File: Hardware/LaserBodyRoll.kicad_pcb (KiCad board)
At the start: 2 copper layers, 104 x 40 mm, 93 parts, among them J1 CONN_01X02, J2 FTSH-105-01-L-DV-K, J3 Conn_01x04, J4 Conn_01x04, J5 CONN_01X02, J6 CONN_01X02, J8 Raspberry_Pi_2_3, Q1 Q_NPN_BCE, Q2 Q_NPN_BCE, Q3 Q_NPN_BCE, Q4 Q_NPN_BCE, U1 TPS821XX, U2 CY8C4A25LQI-473, U3 LMC6032, U5 ICM-20602, U6 VL53L0X, U7 STLM75

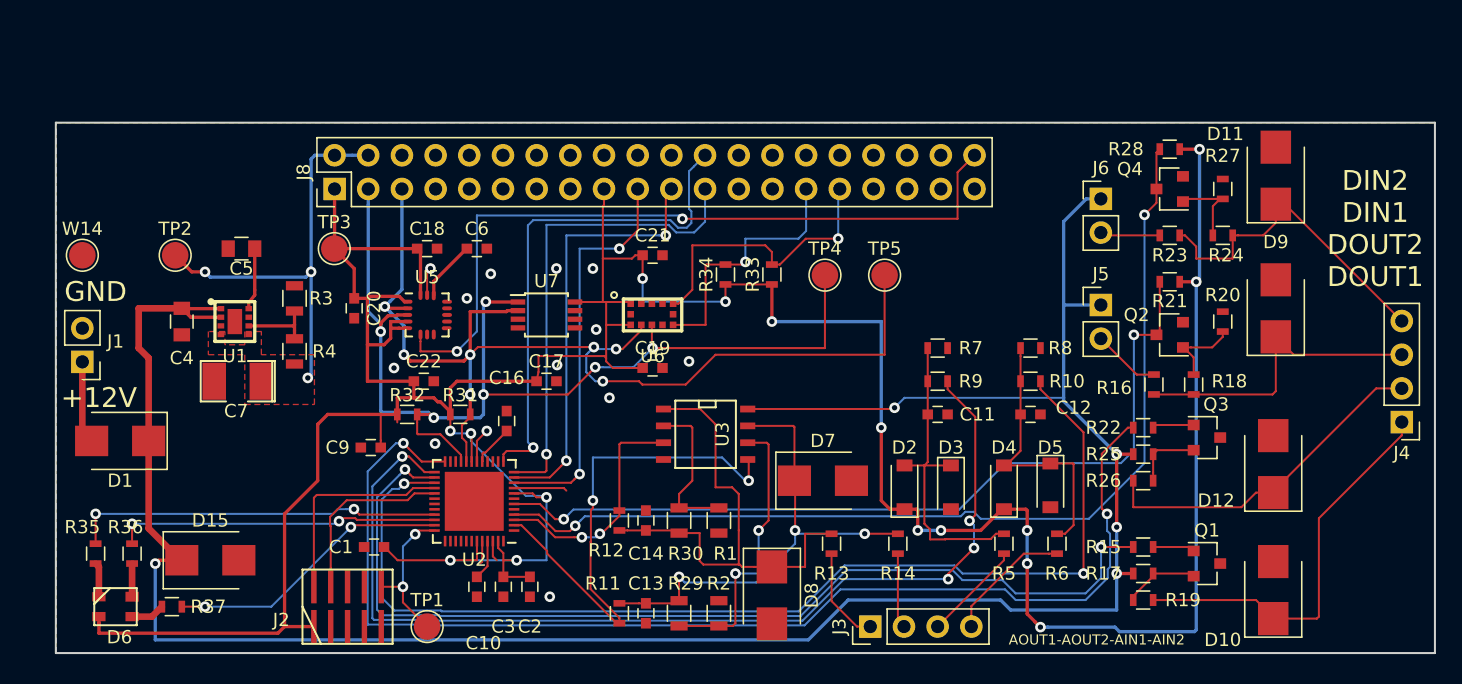
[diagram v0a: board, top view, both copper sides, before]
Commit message: Worked on initial placement.
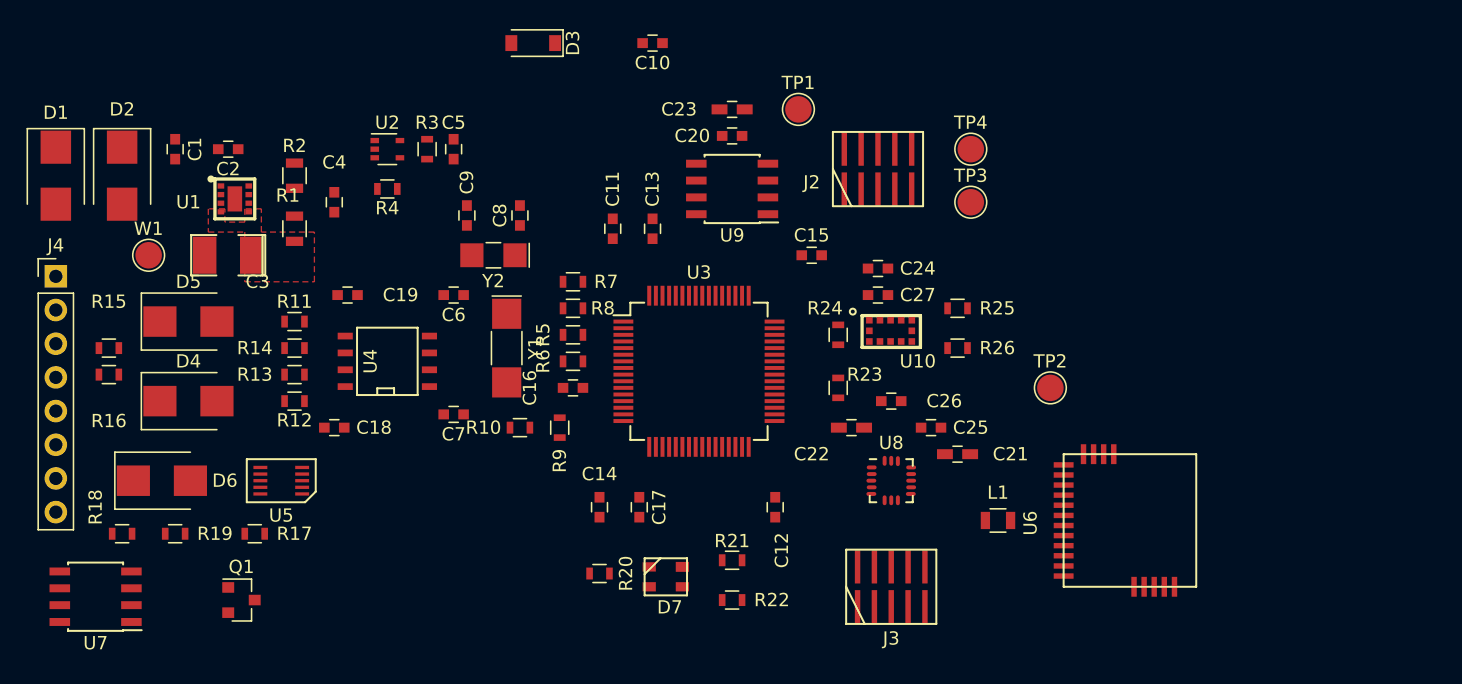
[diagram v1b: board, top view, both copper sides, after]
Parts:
- removed D10, D11, D12, D15, D9: D_TVS, Diodes_SMD:D_SMB
- removed D8: D_Zener, Diodes_SMD:D_SMB
- removed J1, J5, J6: CONN_01X02, Pin_Headers:Pin_Header_Straight_1x02_Pitch2.54mm
- removed J8: Raspberry_Pi_2_3, Pin_Headers:Pin_Header_Straight_2x20_Pitch2.54mm
- removed Q2, Q3, Q4: Q_NPN_BCE, TO_SOT_Packages_SMD:SOT-23
- removed R27: 24.3k, Resistors_SMD:R_0603
- removed R28: 75k, Resistors_SMD:R_0603
- removed R29, R30: 30k, Resistors_SMD:R_0805
- removed R31, R32: 1.7k, Resistors_SMD:R_0603
- removed R33, R34: 10k, Resistors_SMD:R_0603
- removed R35, R36, R37: 330, Resistors_SMD:R_0603
- removed TP5: Test_Point, Connectors_TestPoints:Test_Point_Pad_d2.0mm
- removed W14: TEST_1P, Connectors_TestPoints:Test_Point_Pad_d2.0mm
- added C15: 100n, Capacitors_SMD:C_0603, F.Cu at (97.0, 50.0)
- added C23: 1u, Capacitors_SMD:C_0603_HandSoldering, F.Cu at (91.0, 39.0)
- added C24: 0.1u, Capacitors_SMD:C_0603, F.Cu at (102.0, 51.0)
- added C25: 2.2U, Capacitors_SMD:C_0603, F.Cu at (106.0, 63.0)
- added C26: 10n, Capacitors_SMD:C_0603, F.Cu at (103.0, 61.0)
- added C27: 4.7u, Capacitors_SMD:C_0603, F.Cu at (102.0, 53.0)
- added C8: 6.8, Capacitors_SMD:C_0603, F.Cu at (75.0, 47.0)
- added L1: L_Core_Ferrite, Inductors_SMD:L_0805, F.Cu at (111.0, 70.0)
- added U10: VL53L0X, KicadFootprint:VL53L0x, F.Cu at (103.0, 55.8)
- added U4: LMC6032, SMD_Packages:SOIC-8-N, F.Cu at (65.0, 58.0)
- added U8: ICM-20602, KicadFootprint:QFN-16-no_center_3x3mm_Pitch0.5mm, F.Cu at (103.0, 67.0)
- added U9: W25Qxx, Housings_SOIC:SOIC-8_3.9x4.9mm_Pitch1.27mm, F.Cu at (91.0, 45.0)
- added W1: TEST_1P, Connectors_TestPoints:Test_Point_Pad_d2.0mm, F.Cu at (47.0, 50.0)
- added Y1: 8MHz, Crystals:Crystal_SMD_MicroCrystal_CC4V-T1A-2pin_5.0x1.9mm_HandSoldering, F.Cu at (74.0, 57.0)
- added Y2: 32.768, Crystals:Crystal_SMD_MicroCrystal_CC7V-T1A-2pin_3.2x1.5mm_HandSoldering, F.Cu at (73.0, 50.0)
- C1: value 0.1u -> 10u
- C10: value 0.1u -> 1.5F
- C11: value .01u -> 4.7u
- C12, C13, C14: value .01u -> 100n
- C17: value 0.1u -> 10n
- C18: value 2.2U -> 10n
- C19: value 100n -> 10n
- C2: value 0.1u -> 3.3n
- C20: value 10n -> 0.1n
- C21: value 4.7u -> 0.1u; footprint Capacitors_SMD:C_0603 -> Capacitors_SMD:C_0603_HandSoldering
- C22: footprint Capacitors_SMD:C_0603 -> Capacitors_SMD:C_0603_HandSoldering
- C3: value 1u -> 22u; footprint Capacitors_SMD:C_0603 -> SMD_Packages:SMD-1210_Pol
- C4: value 10u -> 1u; footprint Capacitors_SMD:C_0805 -> Capacitors_SMD:C_0603
- C5: value 3.3n -> 2.2U; footprint Capacitors_SMD:C_0805 -> Capacitors_SMD:C_0603
- C6: value 0.1u -> 20p
- C7: value 22u -> 20p; footprint SMD_Packages:SMD-1210_Pol -> Capacitors_SMD:C_0603
- C9: value 1u -> 6.8
- D2: value D_Zener -> D_TVS; footprint Diodes_SMD:D_SOD-123 -> Diodes_SMD:D_SMB
- D3: value D_Zener -> D
- D4, D5: footprint Diodes_SMD:D_SOD-123 -> Diodes_SMD:D_SMB
- D6: value LED_RABG -> D_TVS; footprint KicadFootprint:CREE_PLCC4 -> Diodes_SMD:D_SMB
- D7: value D_Zener -> LED_RABG; footprint Diodes_SMD:D_SMB -> KicadFootprint:CREE_PLCC4
- J3: value Conn_01x04 -> FTSH-105-01-L-DV-K; footprint Pin_Headers:Pin_Header_Straight_1x04_Pitch2.54mm -> KicadFootprint:FTSH-105-01-L-DV-K
- J4: value Conn_01x04 -> Conn_01x08; footprint Pin_Headers:Pin_Header_Straight_1x04_Pitch2.54mm -> Pin_Headers:Pin_Header_Straight_1x08_Pitch2.54mm
- R1: value 10k -> 525k
- R10: value 24.3k -> 75k
- R11, R12: value DNI -> 24.3k
- R2: value 10k -> 100k
- R20, R22: value 24.3k -> 330
- R21: value 75k -> 330
- R23, R24: value 24.3k -> 1.7k
- R25, R26, R9: value 24.3k -> 10k
- R3: value 100k -> 360; footprint Resistors_SMD:R_0805 -> Resistors_SMD:R_0603
- R4: value 525k -> 120; footprint Resistors_SMD:R_0805 -> Resistors_SMD:R_0603
- R5, R6: value 24.3k -> 0
- R7, R8: value DNI -> 0
- U2: value CY8C4A25LQI-473 -> LDK130-ADJ_SOT23_SOT353; footprint Housings_DFN_QFN:UQFN-48-1EP_6x6mm_Pitch0.4mm -> TO_SOT_Packages_SMD:SOT-353_SC-70-5
- U3: value LMC6032 -> STM32F303RETx; footprint SMD_Packages:SOIC-8-N -> Housings_QFP:TQFP-64_10x10mm_Pitch0.5mm
- U5: value ICM-20602 -> ITS42K5D; footprint KicadFootprint:QFN-16-no_center_3x3mm_Pitch0.5mm -> KicadFootprint:PG-TSON-10
- U6: value VL53L0X -> CYBLE-022001-00; footprint KicadFootprint:VL53L0x -> KicadFootprint:CYBLE-022001
- U7: value STLM75 -> TJA1051T-3; footprint Housings_SSOP:TSSOP-8_3x3mm_Pitch0.65mm -> Housings_SOIC:SOIC-8_3.9x4.9mm_Pitch1.27mm
- moved J4 102.1 mm to (40.0, 51.6), turned to 0 degrees
- moved R18 81.6 mm to (45.0, 71.0), turned to 0 degrees
- moved R15 79.4 mm to (44.0, 57.0), turned to 0 degrees
- moved R16 78.8 mm to (44.0, 59.0), turned to 0 degrees
- moved R19 73.2 mm to (49.0, 71.0), turned to 0 degrees
- moved Q1 72.9 mm to (54.0, 76.0)
- moved R17 67.1 mm to (55.0, 71.0), turned to 0 degrees
- moved TP2 66.8 mm to (115.0, 60.0)
- moved D5 66.2 mm to (50.0, 55.0), turned to 0 degrees
- moved D2 63.5 mm to (45.0, 44.0), turned to 270 degrees
- moved D4 61.8 mm to (50.0, 61.0), turned to 0 degrees
- moved J2 51.9 mm to (102.0, 43.5)
- moved R20 50.7 mm to (81.0, 74.0), turned to 0 degrees
- moved TP3 48.1 mm to (109.0, 46.0)
- moved TP1 48.0 mm to (96.0, 39.0)
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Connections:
- C1 pad 1: VCC -> 12V
- C11 pad 1: Net-(C11-Pad1) -> VCC
- C12 pad 1: Net-(C12-Pad1) -> VCC
- C13 pad 1: Net-(C13-Pad1) -> VCC
- C14 pad 1: Net-(C14-Pad1) -> VCC
- C16 pad 1: Net-(C16-Pad1) -> VCC
- C18 pad 1: VCC -> Net-(C18-Pad1)
- C19 pad 1: VCC -> Net-(C19-Pad1)
- C2 pad 1: VCC -> Net-(C2-Pad1)
- C21 pad 1: VCC -> Net-(C21-Pad1)
- C3 pad 1: VCC -> 5V
- C4 pad 1: /IO/12V -> 5V
- C5 pad 1: Net-(C5-Pad1) -> VCC
- C7 pad 1: +5V -> Net-(C7-Pad1)
- C9 pad 1: VCC -> Net-(C9-Pad1)
- D1 pad 1: /IO/12V -> 12V
- D1 pad 2: Net-(D1-Pad2) -> PWR_IN
- D2 pad 1: VCC -> 12V
- D2 pad 2: Net-(C11-Pad1) -> GND
- D3 pad 1: Net-(C11-Pad1) -> Net-(C10-Pad1)
- D3 pad 2: GND -> VCC
- D4 pad 1: VCC -> Net-(C18-Pad1)
- D4 pad 2: Net-(C12-Pad1) -> GND
- D5 pad 1: Net-(C12-Pad1) -> Net-(C19-Pad1)
- D6 pad 1: Net-(D6-Pad1) -> /IO/DIN
- D6 pad 2: VCC -> GND
- D7 pad 1: Net-(C13-Pad1) -> Net-(D7-Pad1)
- D7 pad 2: GND -> VCC
- J2 pad 10: /Processor/XRES -> /Processor/STM_RES
- J2 pad 2: /Processor/SWDIO -> /Processor/STM_SWDIO
- J2 pad 4: /Processor/SWDCLK -> /Processor/STM_SWDCLK
- J3 pad 1: /IO/ANA_OUT1 -> VCC
- J3 pad 2: /IO/ANA_OUT2 -> /Logic/SWDIO
- J3 pad 3: /IO/ANA_IN1 -> GND
- J3 pad 4: /IO/ANA_IN2 -> /Logic/SWDCLK
- J4 pad 1: /IO/DOUT1 -> PWR_IN
- J4 pad 2: /IO/DOUT2 -> GND
- J4 pad 3: /IO/DIN1 -> /IO/ANA_OUT1
- J4 pad 4: /IO/DIN2 -> /IO/ANA_OUT2
- Q1 pad 2: Net-(Q1-Pad2) -> GND
- Q1 pad 3: GND -> CPU_DIN1
- R1 pad 1: Net-(R1-Pad1) -> 5V
- R1 pad 2: GND -> Net-(R1-Pad2)
- R10 pad 1: /IO/CPU_ANA_IN2 -> 12V
- R10 pad 2: Net-(C12-Pad1) -> Net-(R10-Pad2)
- R11 pad 1: Net-(C13-Pad1) -> Net-(R11-Pad1)
- R11 pad 2: /IO/CPU_ANA_OUT2 -> GND
- R12 pad 1: Net-(C14-Pad1) -> Net-(R12-Pad1)
- R12 pad 2: /IO/CPU_ANA_OUT1 -> GND
- R13 pad 1: /IO/ANA_OUT1 -> Net-(R12-Pad1)
- R13 pad 2: Net-(C14-Pad1) -> Net-(C18-Pad1)
- R14 pad 1: /IO/ANA_OUT2 -> Net-(R11-Pad1)
- R14 pad 2: Net-(C13-Pad1) -> Net-(C19-Pad1)
- R15 pad 1: Net-(Q1-Pad1) -> /IO/ANA_OUT1
- R15 pad 2: /IO/CPU_DOUT1 -> Net-(C19-Pad1)
- R16 pad 1: /IO/DIN1 -> /IO/ANA_OUT2
- R16 pad 2: Net-(J5-Pad2) -> Net-(C18-Pad1)
- R17 pad 1: Net-(Q1-Pad2) -> /IO/DIN
- R17 pad 2: /IO/12V -> /IO/12V_PULLUP
- R18 pad 1: /IO/DIN1 -> /IO/DIN
- R18 pad 2: Net-(Q2-Pad1) -> Net-(Q1-Pad1)
- R19 pad 1: /IO/DOUT1 -> Net-(Q1-Pad1)
- R19 pad 2: Net-(Q1-Pad2) -> GND
- R2 pad 1: Net-(R2-Pad1) -> Net-(R1-Pad2)
- R20 pad 1: Net-(Q2-Pad1) -> Net-(D7-Pad1)
- R20 pad 2: GND -> RED
- R21 pad 1: VCC -> Net-(D7-Pad4)
- R21 pad 2: /IO/CPU_DIN1 -> GREEN
- R22 pad 1: Net-(Q3-Pad1) -> Net-(D7-Pad3)
- R22 pad 2: /IO/CPU_DOUT2 -> BLUE
- R23 pad 1: /IO/DIN2 -> VCC
- R23 pad 2: Net-(J6-Pad2) -> SCL
- R24 pad 1: /IO/DIN2 -> VCC
- R24 pad 2: Net-(Q4-Pad1) -> SDA
- R25 pad 1: Net-(Q3-Pad2) -> VCC
- R25 pad 2: /IO/12V -> /Logic/VL53L0X_XSHUT
- R26 pad 1: /IO/DOUT2 -> VCC
- R26 pad 2: Net-(Q3-Pad2) -> /Logic/VL53L0X_GP
- R3 pad 1: Net-(R3-Pad1) -> VCC
- R3 pad 2: GND -> Net-(R3-Pad2)
- R4 pad 1: +5V -> Net-(R3-Pad2)
- R4 pad 2: Net-(R3-Pad1) -> GND
- R5 pad 1: Net-(C11-Pad1) -> Net-(R5-Pad1)
- R5 pad 2: /IO/ANA_IN1 -> Net-(C6-Pad1)
- R6 pad 1: Net-(C12-Pad1) -> Net-(R6-Pad1)
- R6 pad 2: /IO/ANA_IN2 -> Net-(C7-Pad1)
- R7 pad 1: GND -> Net-(R7-Pad1)
- R7 pad 2: Net-(C11-Pad1) -> Net-(C8-Pad1)
- R8 pad 1: GND -> Net-(R8-Pad1)
- R8 pad 2: Net-(C12-Pad1) -> Net-(C9-Pad1)
- R9 pad 1: /IO/CPU_ANA_IN1 -> GND
- R9 pad 2: Net-(C11-Pad1) -> Net-(R10-Pad2)
- TP1 pad 1: /Processor/XRES -> /Processor/STM_RES
- TP2 pad 1: +5V -> /Logic/XRES
- TP3 pad 1: VCC -> SCL
- TP4 pad 1: /Processor/SDA -> SDA
- U1 pad 1: /IO/12V -> 12V
- U1 pad 2: /IO/12V -> 12V
- U1 pad 4: +5V -> 5V
- U1 pad 5: +5V -> 5V
- U1 pad 6: Net-(R3-Pad1) -> Net-(R1-Pad2)
- U1 pad 8: Net-(C5-Pad1) -> Net-(C2-Pad1)
- U2 pad 1: Net-(U2-Pad1) -> 5V
- U2 pad 2: /IO/CPU_ANA_OUT2 -> GND
- U2 pad 3: /IO/CPU_ANA_OUT1 -> 5V
- U2 pad 4: /IO/CPU_DIN2 -> Net-(R3-Pad2)
- U2 pad 5: Net-(U2-Pad5) -> VCC
- U3 pad 1: Net-(C14-Pad1) -> Net-(C10-Pad1)
- U3 pad 2: Net-(R1-Pad1) -> Net-(U3-Pad2)
- U3 pad 3: /IO/CPU_ANA_OUT1 -> Net-(R7-Pad1)
- U3 pad 4: GND -> Net-(R8-Pad1)
- U3 pad 5: /IO/CPU_ANA_OUT2 -> Net-(R5-Pad1)
- U3 pad 6: Net-(R2-Pad1) -> Net-(R6-Pad1)
- U3 pad 7: Net-(C13-Pad1) -> /Processor/STM_RES
- U3 pad 8: /IO/12V -> CPU_DOUT1
- U5 pad 1: VCC -> CPU_DOUT1
- U5 pad 2: /Processor/SCL -> CPU_DOUT1_ST
- U5 pad 3: /Processor/SDA -> GND
- U5 pad 4: VCC -> CPU_DOUT2
- U5 pad 5: VCC -> CPU_DOUT2_ST
- U5 pad 6: /Processor/ICM_INT -> GND
- U5 pad 7: Net-(U5-Pad7) -> /IO/12V_PULLUP
- U5 pad 8: Net-(U5-Pad8) -> 12V
- U5 pad 9: GND -> /IO/DOUT
- U6 pad 1: VCC -> GND
- U6 pad 10: /Processor/SCL -> GND
- U6 pad 11: VCC -> /Logic/SWDIO
- U6 pad 12: GND -> BLE_SCLK
- U6 pad 2: GND -> Net-(U6-Pad2)
- U6 pad 3: GND -> Net-(U6-Pad3)
- U6 pad 4: GND -> Net-(U6-Pad4)
- U6 pad 5: /Processor/VL53L0X_XSHUT -> Net-(L1-Pad2)
- U6 pad 6: GND -> BLE_CS
- U6 pad 7: /Processor/VL53L0X_GP -> /Logic/SWDCLK
- U6 pad 9: /Processor/SDA -> Net-(U6-Pad9)
- U7 pad 1: /Processor/SDA -> CAN_TXD
- U7 pad 2: /Processor/SCL -> GND
- U7 pad 3: Net-(U7-Pad3) -> 5V
- U7 pad 4: GND -> CAN_RXD
- U7 pad 5: GND -> VCC
- U7 pad 6: GND -> CANL
- U7 pad 7: GND -> CANH
- U7 pad 8: VCC -> GND
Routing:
- net VCC: track 285.9 -> 0.00 mm, vias 16 -> 0
- net /IO/12V: track 175.7 -> 0.00 mm, vias 5 -> 0
- net /IO/CPU_DOUT2: track 89.7 -> 0.00 mm, vias 2 -> 0
- net /IO/CPU_ANA_IN2: track 82.8 -> 0.00 mm, vias 2 -> 0
- net /Processor/SCL: track 82.3 -> 0.00 mm, vias 7 -> 0
- net /Processor/SDA: track 80.8 -> 0.00 mm, vias 6 -> 0
- net /IO/CPU_ANA_IN1: track 77.8 -> 0.00 mm, vias 4 -> 0
- net /IO/CPU_DOUT1: track 76.1 -> 0.00 mm, vias 2 -> 0
- net /IO/CPU_DIN2: track 74.8 -> 0.00 mm, vias 2 -> 0
- net /IO/CPU_DIN1: track 63.9 -> 0.00 mm, vias 2 -> 0
- net /Processor/ICM_INT: track 56.6 -> 0.00 mm, vias 2 -> 0
- net /IO/CPU_ANA_OUT2: track 39.1 -> 0.00 mm, vias 2 -> 0
- net /Processor/SS: track 38.5 -> 0.00 mm, vias 1 -> 0
- net Net-(C14-Pad1): track 37.3 -> 0.00 mm
- net Net-(C13-Pad1): track 36.8 -> 0.00 mm, vias 3 -> 0
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- removed copper zone on B.Cu, net GND
- removed copper zone on F.Cu, net GND
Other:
- board outline removed
- board text removed: "+12V"
- board text removed: "AOUT1-AOUT2-AIN1-AIN2"
- board text removed: "DIN2 DIN1 DOUT2 DOUT1"
- board text removed: "GND"
